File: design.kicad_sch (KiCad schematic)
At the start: 84 parts, among them IC1 LM66200DRLR, J1 2601-3108, J10 Conn_01x04, J11 Conn_01x04, J13 Conn_01x03, J14 BM04B-SRSS-TB_LF__SN_, J2 2601-3108, J3 2601-3108, J4 TYPE-C-31-M-12, J5 SKEDD-UPDI-4, J6 Conn_01x04, J7 Conn_01x04, J8 Conn_01x04, J9 Conn_01x04, Q1 AO3400A, Q2 AO3400A, SW1 K3-2235S-K1, U1 ATtiny1616-S, U2 AP2112K-3.3, U4 ATtiny1616-M, U5 CH340K

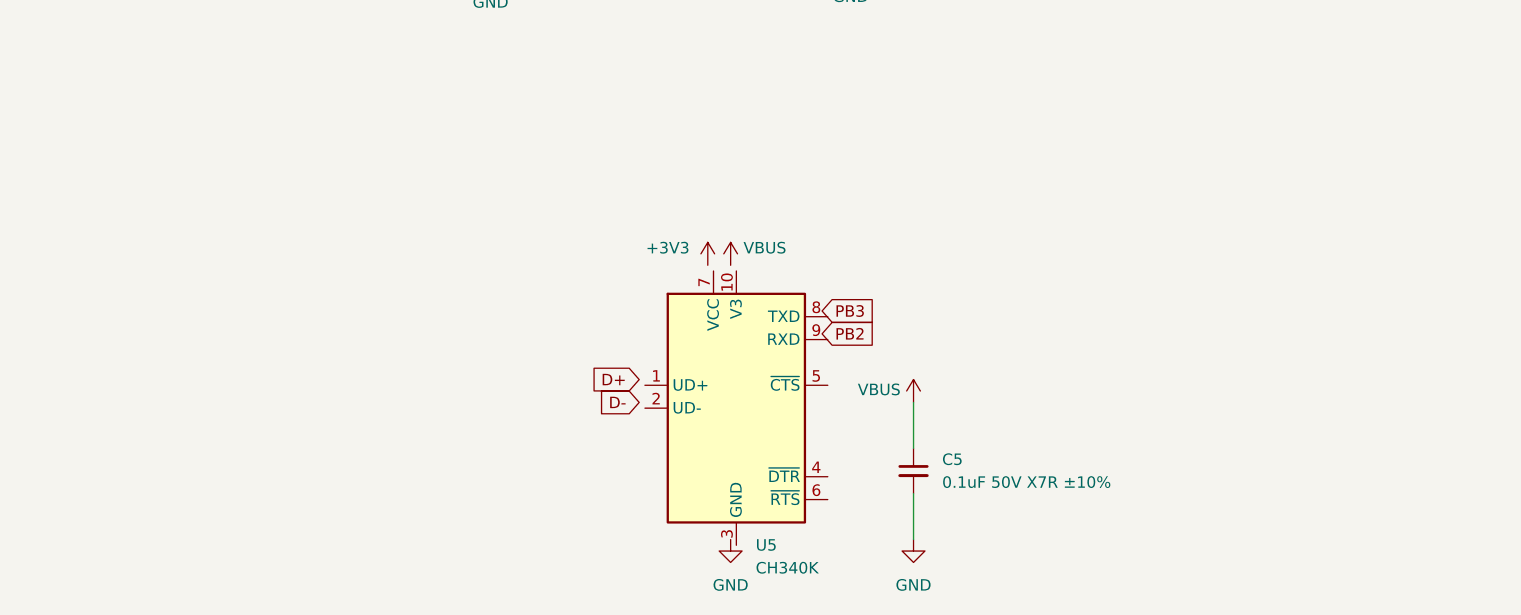
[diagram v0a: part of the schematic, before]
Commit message: Update design.kicad_sch
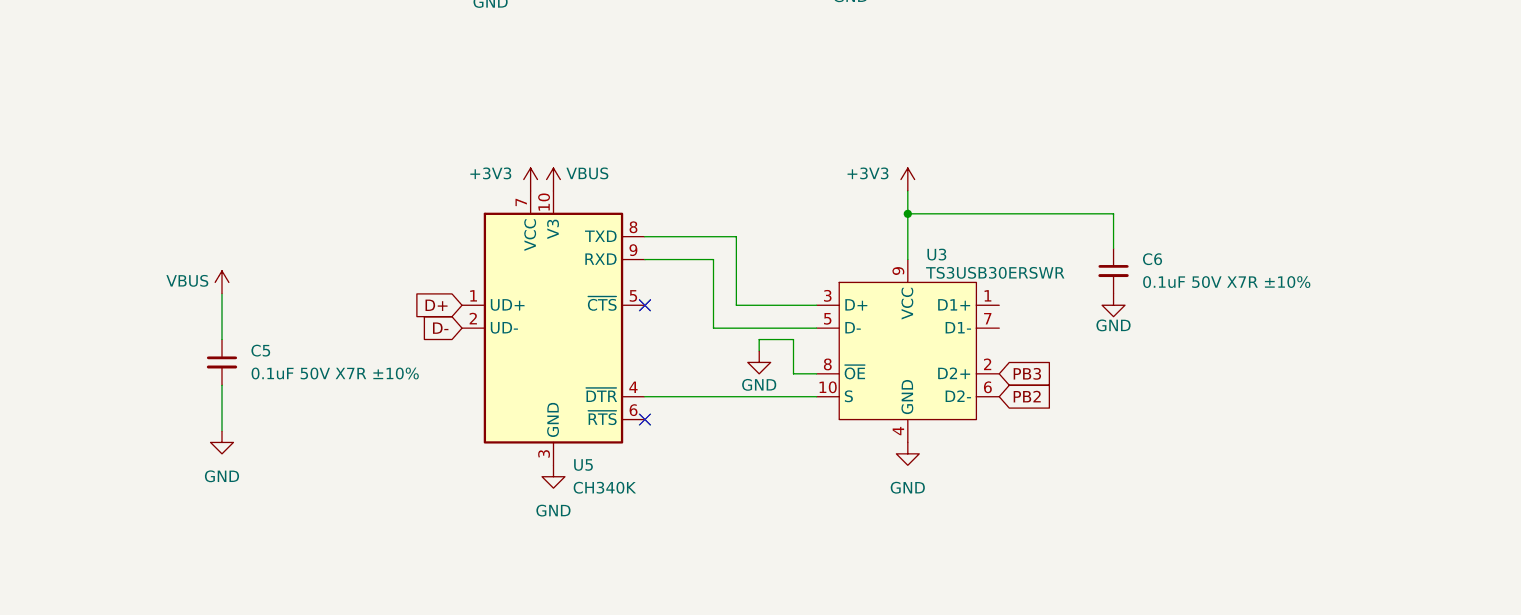
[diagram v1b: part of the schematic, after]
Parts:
- added C6: 0.1uF 50V X7R ±10%, Capacitor_SMD:C_0805_2012Metric, symbol Device:C_Small
- added U3: TS3USB30ERSWR, Package_DFN_QFN:UQFN-10_1.4x1.8mm_P0.4mm, symbol Interface_USB:TS3USB30ERSWR
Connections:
- net +3V3: now also U5.7 (VCC), C6.1, U3.9 (VCC)
- net D+: now also U5.1 (UD+)
- net D-: now also U5.2 (UD-)
- net GND: now also U5.11 (GND), U5.3 (GND), C6.2, U3.4 (GND), U3.8 (~{OE})
- net PB2: now also U3.6 (D2-)
- net PB3: now also U3.2 (D2+)
- net VBUS: now also U5.10 (V3)
- net at U5.4 (~{DTR}): now also U3.10 (S)
- net at U5.8 (TXD): now also U3.3 (D+)
- net at U5.9 (RXD): now also U3.5 (D-)
- no-connect marks 4 -> 6
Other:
- moved on the sheet: C5, U5
